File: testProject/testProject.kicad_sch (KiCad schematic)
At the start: 12 parts

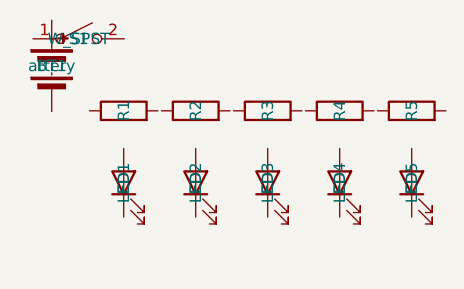
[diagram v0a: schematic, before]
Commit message: exit
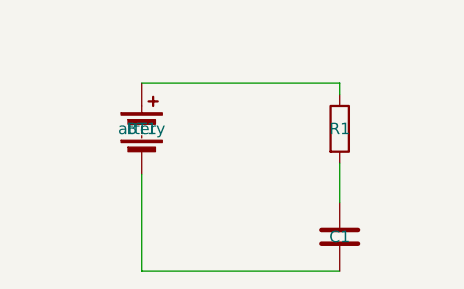
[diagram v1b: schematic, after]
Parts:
- removed LED1, LED2, LED3, LED4, LED5: ED, symbol Device:LED
- removed R2, R3, R4, R5: (no value), symbol Device:R
- removed S1: W_SPST, symbol Switch:SW_SPST
- added C1: (no value), symbol Device:C
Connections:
- net at BT1.1 (+): now also R1.1
- net at BT1.2 (-): now also C1.2
- net at R1.2: now also C1.1

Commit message: removed unneccessary files, clean up notebook
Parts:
- removed BT1: attery, symbol Device:Battery
- removed C1: (no value), symbol Device:C
- removed R1: (no value), symbol Device:R
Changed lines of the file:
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@@
 	(generator_version "8.0")
 	(paper "A4")
- (wire
-		(pts
-			(xy 42 14.92) (xy 42 16.19)
-		)
-		(stroke
-			(width 0)
-			(type default)
-		)
-	)
- (wire
-		(pts
-			(xy 20 14.92) (xy 42 14.92)
-		)
-		(stroke
-			(width 0)
-			(type default)
-		)
-	)
- (wire
-		(pts
-			(xy 42 23.81) (xy 42 28.19)
-		)
-		(stroke
-			(width 0)
-			(type default)
-		)
-	)
- (wire
-		(pts
-			(xy 20 35.81) (xy 20 25.08)
-		)
-		(stroke
-			(width 0)
-			(type default)
-		)
-	)
- (wire
-		(pts
-			(xy 42 35.81) (xy 20 35.81)
-		)
-		(stroke
-			(width 0)
-			(type default)
-		)
-	)
-(symbol
-        (lib_id "Device:C")
-        (at 42 32 0)
-        (unit 1)
-        (exclude_from_sim no)
-        (in_bom yes)
-        (on_board yes)
-        (dnp no)
-        (fields_autoplaced yes)
-        (property "Reference" "C1"
-            (at 42 32 0)
-            (effects
-                (font
-                    (size 1.27 1.27)
-                )
-            )
-        )
-        (property "Value" ""
-            (at 42 32 0)
-            (effects
-                (font
-                    (size 1.27 1.27)
-                )
-            )
-        )
-        (property "Footprint" ""
-            (at 42 32 0)
-            (effects
-                (font
-                    (size 1.27 1.27)
-                )
-                (hide yes)
-            )
-        )
-        (property "Datasheet" "~"
-            (at 42 32 0)
-            (effects
-                (font
-                    (size 1.27 1.27)
-                )
-                (hide yes)
-            )
-        )
-        (property "Description" "npolarized capacitor"
-            (at 42 32 0)
-            (effects
-                (font
-                    (size 1.27 1.27)
-                )
-                (hide yes)
-            )
-        )
-        (pin "1")
-        (pin "2")
-        (instances
-            (project "temp_dea647a7-e0d8-45e4-9bce-23c7e387cf2b"
-                (path "/dea647a7-e0d8-45e4-9bce-23c7e387cf2b"
-                    (reference "C1")
-                    (unit 1)
-                )
-            )
-        )
-    )
-(symbol
-        (lib_id "Device:R")
-        (at 42 20 0)
-        (unit 1)
-        (exclude_from_sim no)
-        (in_bom yes)
-        (on_board yes)
-        (dnp no)
-        (fields_autoplaced yes)
-        (property "Reference" "R1"
-            (at 42 20 0)
-            (effects
-                (font
-                    (size 1.27 1.27)
-                )
-            )
-        )
-        (property "Value" ""
-            (at 42 20 0)
-            (effects
-                (font
-                    (size 1.27 1.27)
-                )
-            )
-        )
-        (property "Footprint" ""
-            (at 42 20 0)
-            (effects
-                (font
-                    (size 1.27 1.27)
-                )
-                (hide yes)
-            )
-        )
-        (property "Datasheet" "~"
-            (at 42 20 0)
-            (effects
-                (font
-                    (size 1.27 1.27)
-                )
-                (hide yes)
-            )
-        )
-        (property "Description" "esistor"
-            (at 42 20 0)
-            (effects
-                (font
-                    (size 1.27 1.27)
-                )
-                (hide yes)
-            )
-        )
-        (pin "1")
-        (pin "2")
-        (instances
-            (project "temp_dea647a7-e0d8-45e4-9bce-23c7e387cf2b"
-                (path "/dea647a7-e0d8-45e4-9bce-23c7e387cf2b"
-                    (reference "R1")
-                    (unit 1)
-                )
-            )
-        )
-    )
-(symbol
-        (lib_id "Device:Battery")
-        (at 20 20 0)
-        (unit 1)
-        (exclude_from_sim no)
-        (in_bom yes)
-        (on_board yes)
-        (dnp no)
-        (fields_autoplaced yes)
-        (property "Reference" "BT1"
-            (at 20 20 0)
-            (effects
-                (font
-                    (size 1.27 1.27)
-                )
-            )
-        )
-        (property "Value" "attery"
-            (at 20 20 0)
-            (effects
-                (font
-                    (size 1.27 1.27)
-                )
-            )
-        )
-        (property "Footprint" ""
-            (at 20 20 0)
-            (effects
-                (font
-                    (size 1.27 1.27)
-                )
-                (hide yes)
-            )
-        )
-        (property "Datasheet" "~"
-            (at 20 20 0)
-            (effects
-                (font
-                    (size 1.27 1.27)
-                )
-                (hide yes)
-            )
-        )
-        (property "Description" "ultiple-cell battery"
-            (at 20 20 0)
-            (effects
-                (font
-                    (size 1.27 1.27)
-                )
-                (hide yes)
-            )
-        )
-        (pin "1")
-        (pin "2")
-        (instances
-            (project "temp_dea647a7-e0d8-45e4-9bce-23c7e387cf2b"
-                (path "/dea647a7-e0d8-45e4-9bce-23c7e387cf2b"
-                    (reference "BT1")
-                    (unit 1)
-                )
-            )
-        )
-    )
- 	(sheet_instances
+	(sheet_instances
 		(path "/"
 			(page "1")
